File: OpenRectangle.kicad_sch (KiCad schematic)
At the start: 21 parts, among them J1 RPI_PICO-TH, SW1 MX_SW_HS, SW10 MX_SW_HS, SW11 MX_SW_HS, SW12 MX_SW_HS, SW13 MX_SW_HS, SW14 MX_SW_HS, SW15 MX_SW_HS, SW16 MX_SW_HS, SW17 MX_SW_HS, SW18 MX_SW_HS, SW19 MX_SW_HS, SW2 MX_SW_HS, SW20 MX_SW_HS, SW3 MX_SW_HS, SW4 MX_SW_HS, SW5 MX_SW_HS, SW6 MX_SW_HS, SW7 MX_SW_HS, SW8 MX_SW_HS, SW9 MX_SW_HS

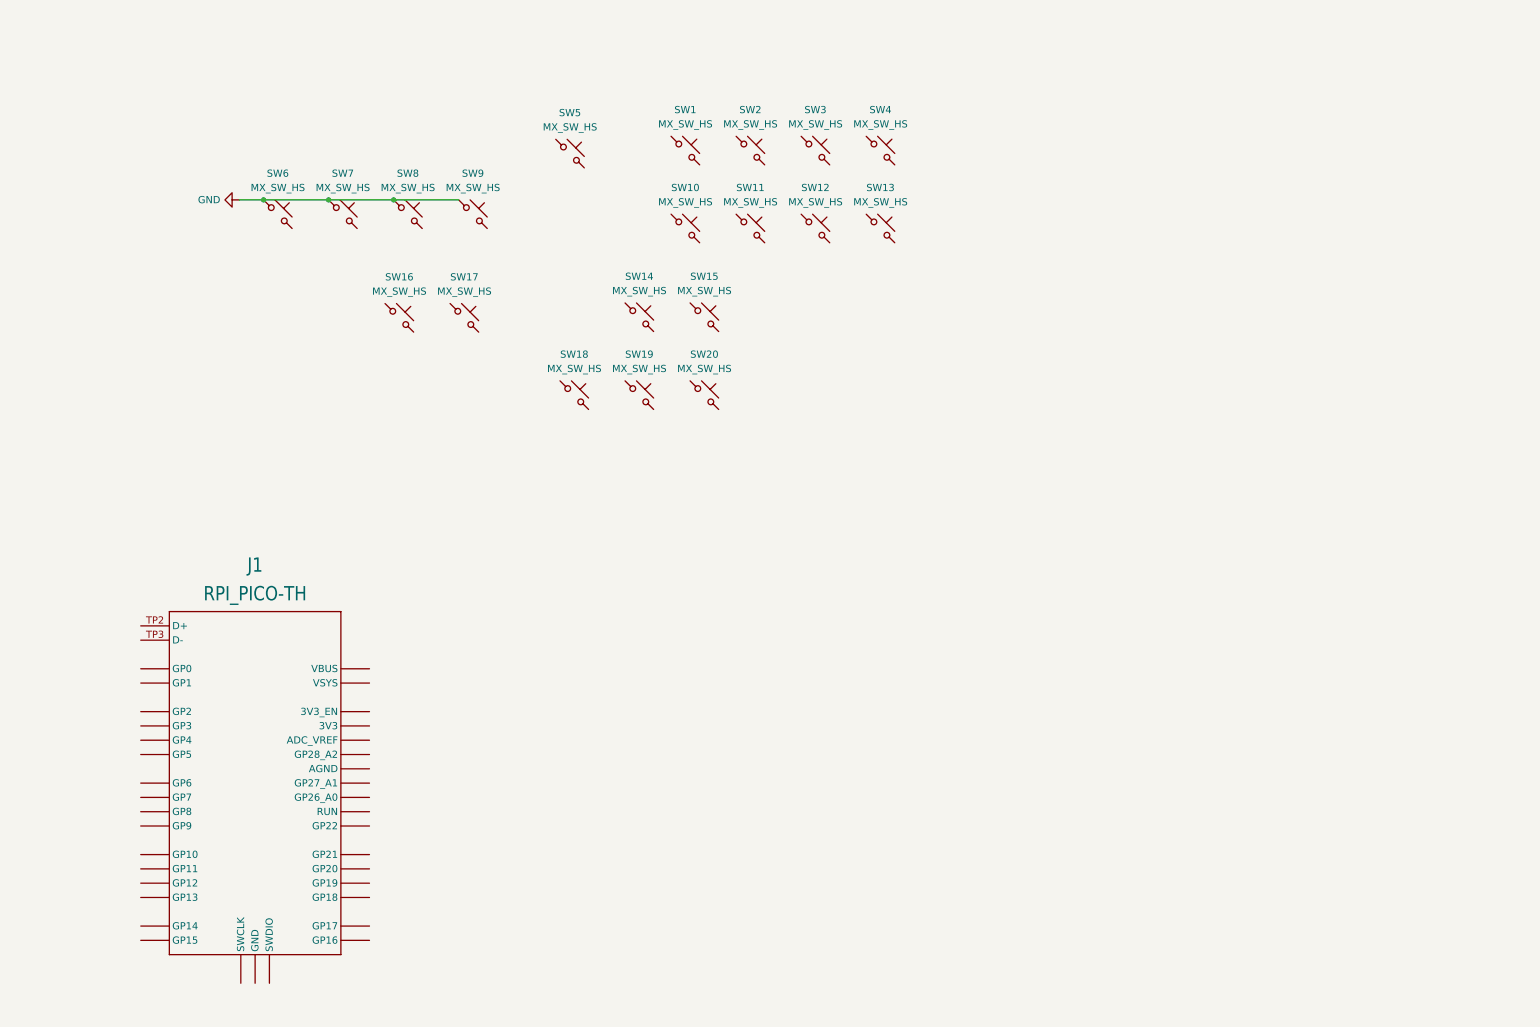
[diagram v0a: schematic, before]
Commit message: Técnicamente ya funciona
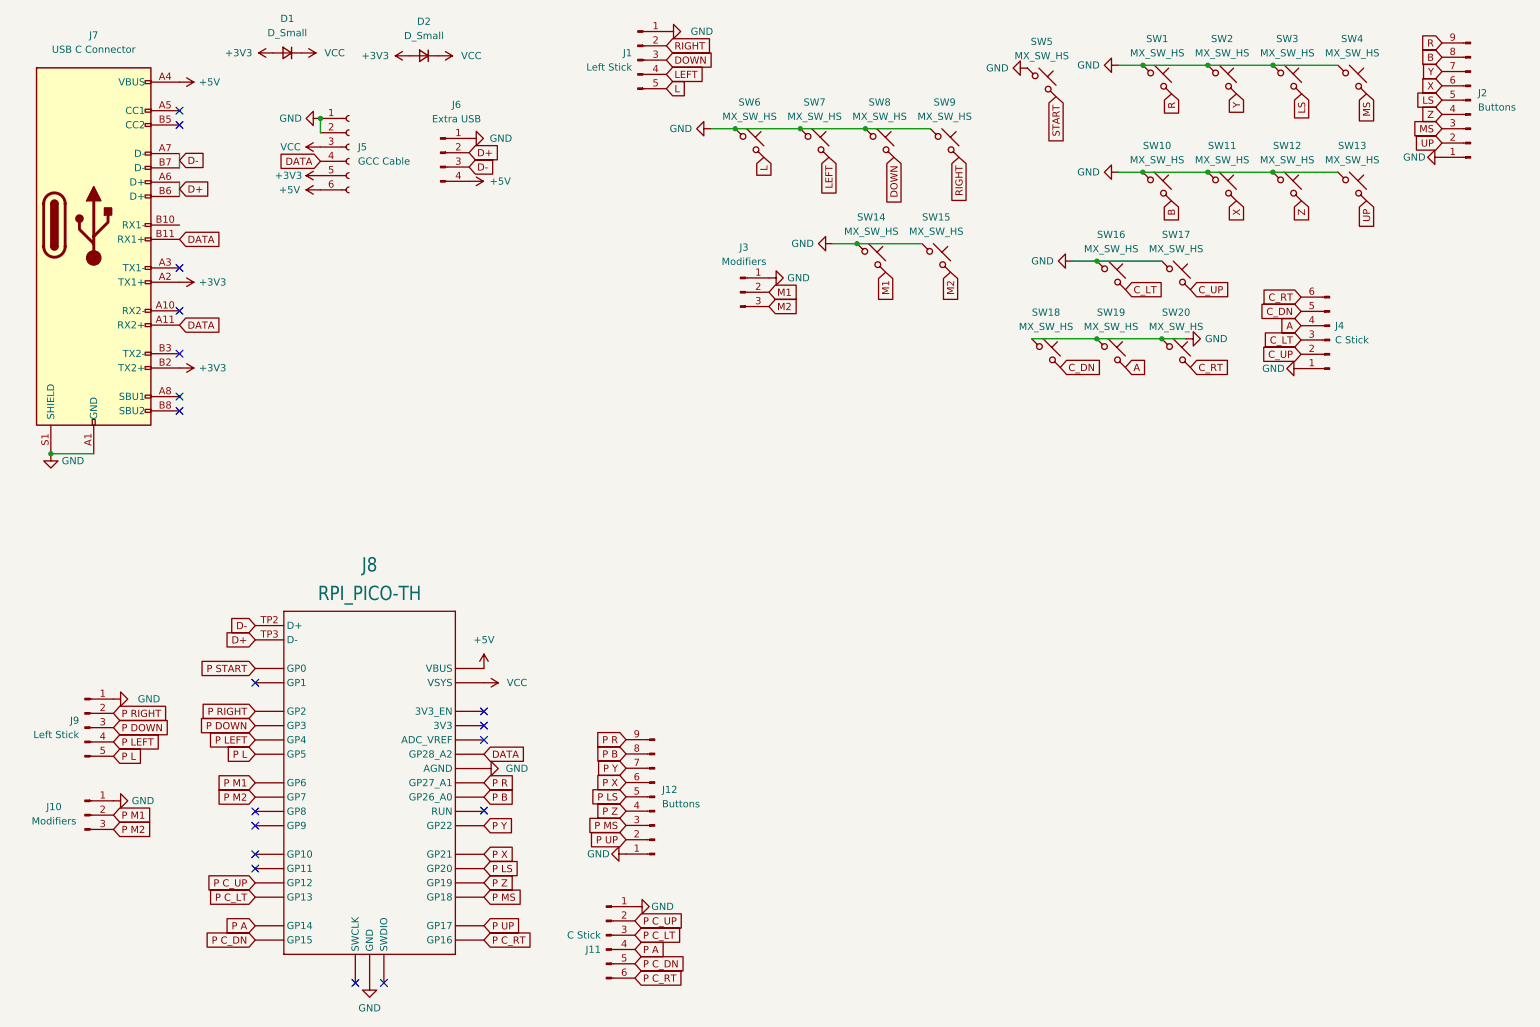
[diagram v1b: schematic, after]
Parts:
- added D1: D_Small, Diode_THT:D_DO-41_SOD81_P10.16mm_Horizontal, symbol Device:D_Small
- added D2: D_Small, Diode_SMD:D_0805_2012Metric, symbol Device:D_Small
- added J1, J9: Left Stick, Connector_PinHeader_2.54mm:PinHeader_1x05_P2.54mm_Vertical, symbol Connector:Conn_01x05_Male
- added J10, J3: Modifiers, Connector_PinHeader_2.54mm:PinHeader_1x03_P2.54mm_Vertical, symbol Connector:Conn_01x03_Male
- added J11, J4: C Stick, Connector_PinHeader_2.54mm:PinHeader_1x06_P2.54mm_Vertical, symbol Connector:Conn_01x06_Male
- added J12, J2: Buttons, Connector_PinHeader_2.54mm:PinHeader_1x09_P2.54mm_Vertical, symbol Connector:Conn_01x09_Male
- added J5: GCC Cable, Connector_PinHeader_2.54mm:PinHeader_1x06_P2.54mm_Vertical, symbol Connector:Conn_01x06_Female
- added J6: Extra USB, Connector_PinHeader_2.54mm:PinHeader_1x04_P2.54mm_Vertical, symbol Connector:Conn_01x04_Male
- added J7: USB C Connector, Connector_USB:USB_C_Receptacle_Amphenol_12401548E4-2A, symbol Connector:USB_C_Receptacle
- renumbered J1 to J8, SW16 to SW14, SW17 to SW15, SW14 to SW16, SW15 to SW17
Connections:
- net GND: now also J8.AGND, J8.GND@1 (GND), J8.GND@2 (GND), J8.GND@3 (GND), J8.GND@4 (GND), J8.GND@5 (GND), J8.GND@6 (GND), J8.GND@7 (GND), J8.GND@8 (GND), SW1.1, SW10.1, SW11.1, SW12.1, SW13.1, SW14.1, SW15.1, SW16.1, SW17.1, SW18.1, SW19.1, SW2.1, SW20.1, SW3.1, SW4.1, SW5.1, J1.1 (Pin_1), J10.1 (Pin_1), J11.1 (Pin_1), J12.1 (Pin_1), J2.1 (Pin_1), J3.1 (Pin_1), J4.1 (Pin_1), J5.1 (Pin_1), J5.2 (Pin_2), J6.1 (Pin_1), J7.A1 (GND), J7.A12 (GND), J7.B1 (GND), J7.B12 (GND), J7.S1 (SHIELD), J9.1 (Pin_1)
- net C_RT: now reaches SW20.2
- net C_RT: now also J4.6 (Pin_6)
- net M2: now reaches SW15.2
- net M2: now also J3.3 (Pin_3)
- net DOWN: now reaches SW8.2
- net DOWN: now also J1.3 (Pin_3)
- net LEFT: now reaches SW7.2
- net LEFT: now also J1.4 (Pin_4)
- net P START: now reaches J8.GP0
- net P C_UP: now reaches J8.GP12
- net P C_UP: now also J11.2 (Pin_2)
- net P C_LT: now reaches J8.GP13
- net P C_LT: now also J11.3 (Pin_3)
- net P A: now reaches J8.GP14
- net P A: now also J11.4 (Pin_4)
- net P C_DN: now reaches J8.GP15
- net P C_DN: now also J11.5 (Pin_5)
- net P C_RT: now reaches J8.GP16
- net P C_RT: now also J11.6 (Pin_6)
- net P UP: now reaches J8.GP17
- net P UP: now also J12.2 (Pin_2)
- net P MS: now reaches J8.GP18
- net P MS: now also J12.3 (Pin_3)
- net P Z: now reaches J8.GP19
- net P Z: now also J12.4 (Pin_4)
- net P RIGHT: now reaches J8.GP2
- net P RIGHT: now also J9.2 (Pin_2)
- net P LS: now reaches J8.GP20
- net P LS: now also J12.5 (Pin_5)
- net P X: now reaches J8.GP21
- net P X: now also J12.6 (Pin_6)
- net P Y: now reaches J8.GP22
- net P Y: now also J12.7 (Pin_7)
- net P B: now reaches J8.GP26_A0
- net P B: now also J12.8 (Pin_8)
- net P R: now reaches J8.GP27_A1
- net P R: now also J12.9 (Pin_9)
- net DATA: now reaches J8.GP28_A2
- net DATA: now also J5.4 (Pin_4), J7.A11 (RX2+), J7.B11 (RX1+)
- net P DOWN: now reaches J8.GP3
- net P DOWN: now also J9.3 (Pin_3)
- net P LEFT: now reaches J8.GP4
- net P LEFT: now also J9.4 (Pin_4)
- net P L: now reaches J8.GP5
- net P L: now also J9.5 (Pin_5)
- net P M1: now reaches J8.GP6
- net P M1: now also J10.2 (Pin_2)
- net P M2: now reaches J8.GP7
- net P M2: now also J10.3 (Pin_3)
- net D-: now reaches J8.TP2 (D+)
- net D-: now also J6.3 (Pin_3), J7.A7 (D-), J7.B7 (D-)
- net D+: now reaches J8.TP3 (D-)
- net D+: now also J6.2 (Pin_2), J7.A6 (D+), J7.B6 (D+)
- net +5V: now reaches J8.VBUS
- net +5V: now also J5.6 (Pin_6), J6.4 (Pin_4), J7.A4 (VBUS), J7.A9 (VBUS), J7.B4 (VBUS), J7.B9 (VBUS)
- net VCC: now reaches J8.VSYS
- net VCC: now also D1.1 (K), D2.1 (K), J5.3 (Pin_3)
- net Z: now reaches SW12.2
- net Z: now also J2.4 (Pin_4)
- net B: now reaches SW10.2
- net B: now also J2.8 (Pin_8)
- net Y: now reaches SW2.2
- net Y: now also J2.7 (Pin_7)
- net L: now reaches SW6.2
- net L: now also J1.5 (Pin_5)
- net X: now reaches SW11.2
- net X: now also J2.6 (Pin_6)
- net LS: now reaches SW3.2
- net LS: now also J2.5 (Pin_5)
- net R: now reaches SW1.2
- net R: now also J2.9 (Pin_9)
- net UP: now reaches SW13.2
- net UP: now also J2.2 (Pin_2)
- net MS: now reaches SW4.2
- net MS: now also J2.3 (Pin_3)
- net RIGHT: now reaches SW9.2
- net RIGHT: now also J1.2 (Pin_2)
- net M1: now reaches SW14.2
- net M1: now also J3.2 (Pin_2)
- net C_DN: now reaches SW18.2
- net C_DN: now also J4.5 (Pin_5)
- net START: now reaches SW5.2
- net C_UP: now reaches SW17.2
- net C_UP: now also J4.2 (Pin_2)
- net A: now reaches SW19.2
- net A: now also J4.4 (Pin_4)
- net C_LT: now reaches SW16.2
- net C_LT: now also J4.3 (Pin_3)
- new net +3V3: D1.2 (A), D2.2 (A), J5.5 (Pin_5), J7.A2 (TX1+), J7.B2 (TX2+)
- no-connect marks 0 -> 18
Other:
- moved on the sheet: J8, SW1, SW10, SW11, SW12, SW13, SW14, SW15, SW16, SW17, SW18, SW19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
